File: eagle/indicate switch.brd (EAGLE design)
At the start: 71.1 x 54.3 mm, 13 parts, among them IC1 SCT2026CSSG-1, IC2 SCT2026CSSG-1

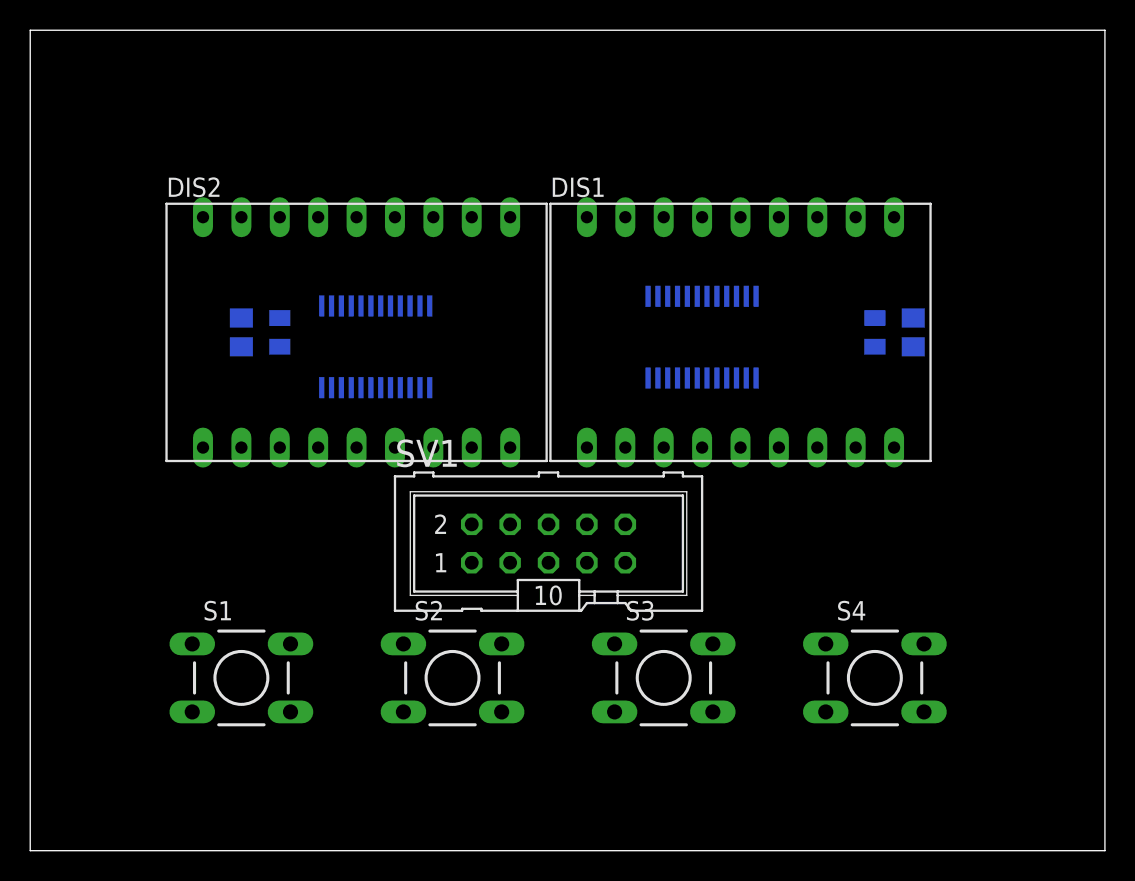
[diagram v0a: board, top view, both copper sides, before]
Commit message: Add files via upload
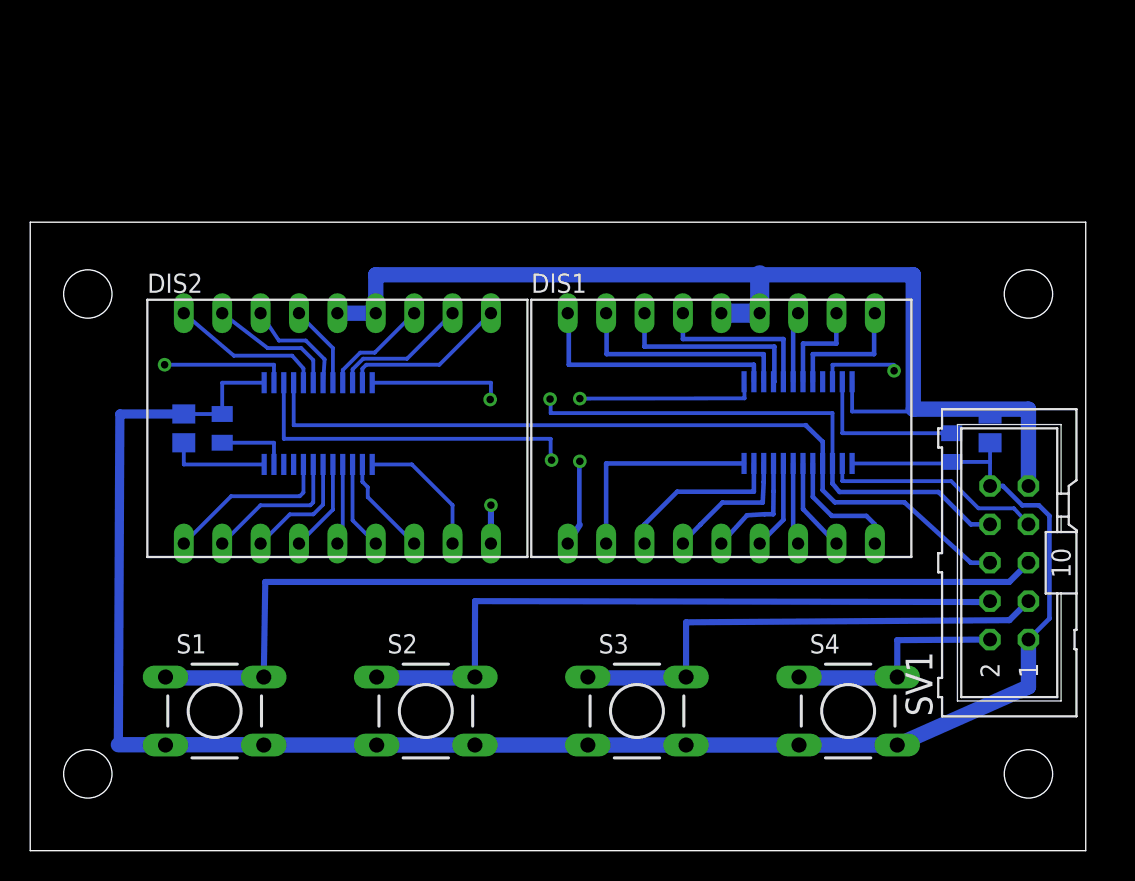
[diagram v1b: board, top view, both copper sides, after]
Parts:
- moved SV1 30.5 mm to (64.8, 19.1), turned to 90 degrees
- moved R1 9.16 mm to (61.0, 26.7)
- moved IC1 8.50 mm to (50.8, 28.6)
- moved C2 8.13 mm to (63.5, 27.9)
- moved R2 7.41 mm to (12.7, 27.9)
- moved C1 7.41 mm to (10.2, 27.9)
- moved DIS1 6.48 mm to (45.7, 27.9)
- moved DIS2 6.48 mm to (20.3, 27.9)
- moved IC2 6.35 mm to (19.1, 27.9)
- moved S4 2.82 mm to (54.1, 9.24)
- moved S1 2.82 mm to (12.2, 9.24)
- moved S2 2.82 mm to (26.2, 9.24)
- moved S3 2.82 mm to (40.1, 9.24)
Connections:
- removed net N$7: C1.1, C2.1, IC1.1, IC2.1, R1.1, R2.1, SV1.9
- net N$1: now also S2.2; no longer S1.2
- net N$12: now also S3.2, SV1.3; no longer IC1.2, SV1.1
- net N$13: now also SV1.8; no longer SV1.2
- net N$14: now also SV1.6; no longer SV1.3
- net N$19: now also DIS1.6
- net N$2: now also S1.2; no longer S2.2
- net N$3: now also S4.2, SV1.2; no longer S3.2, SV1.6
- net N$4: now also IC1.2; no longer S4.2
- net N$5: now also C1.1, C2.1, IC1.1, IC2.1, R1.1, R2.1, SV1.1, SV1.10; no longer SV1.8
- net N$6: now also SV1.9; no longer SV1.10
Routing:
- net N$5: track 0.00 -> 125.0 mm
- net N$6: track 0.00 -> 78.6 mm
- net N$13: track 0.00 -> 58.6 mm
- net N$2: track 0.00 -> 57.3 mm
- net N$14: track 0.00 -> 54.4 mm
- net N$1: track 0.00 -> 39.1 mm
- net N$12: track 0.00 -> 26.8 mm
- net N$24: track 0.00 -> 17.7 mm
- net N$25: track 0.00 -> 16.8 mm
- net N$26: track 0.00 -> 15.0 mm
- net N$4: track 0.00 -> 14.7 mm
- net N$23: track 0.00 -> 14.4 mm
- net N$15: track 0.00 -> 13.6 mm
- net N$27: track 0.00 -> 13.2 mm
- net N$39: track 0.00 -> 11.4 mm
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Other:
- board size 71.1 x 54.3 mm -> 69.8 x 41.6 mm
